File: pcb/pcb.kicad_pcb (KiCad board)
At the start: 2 copper layers, 49 x 31 mm, 37 parts, among them J1 Conn_02x08_Odd_Even, J2 B2B-PH-K-S_LF__SN_, J3 USB_C_Receptacle, J4 Conn_01x04, Q1 MMUN2211LT1G, SW1 SW_SPST, U1 TPS61090, U2 MCP73871-1AA

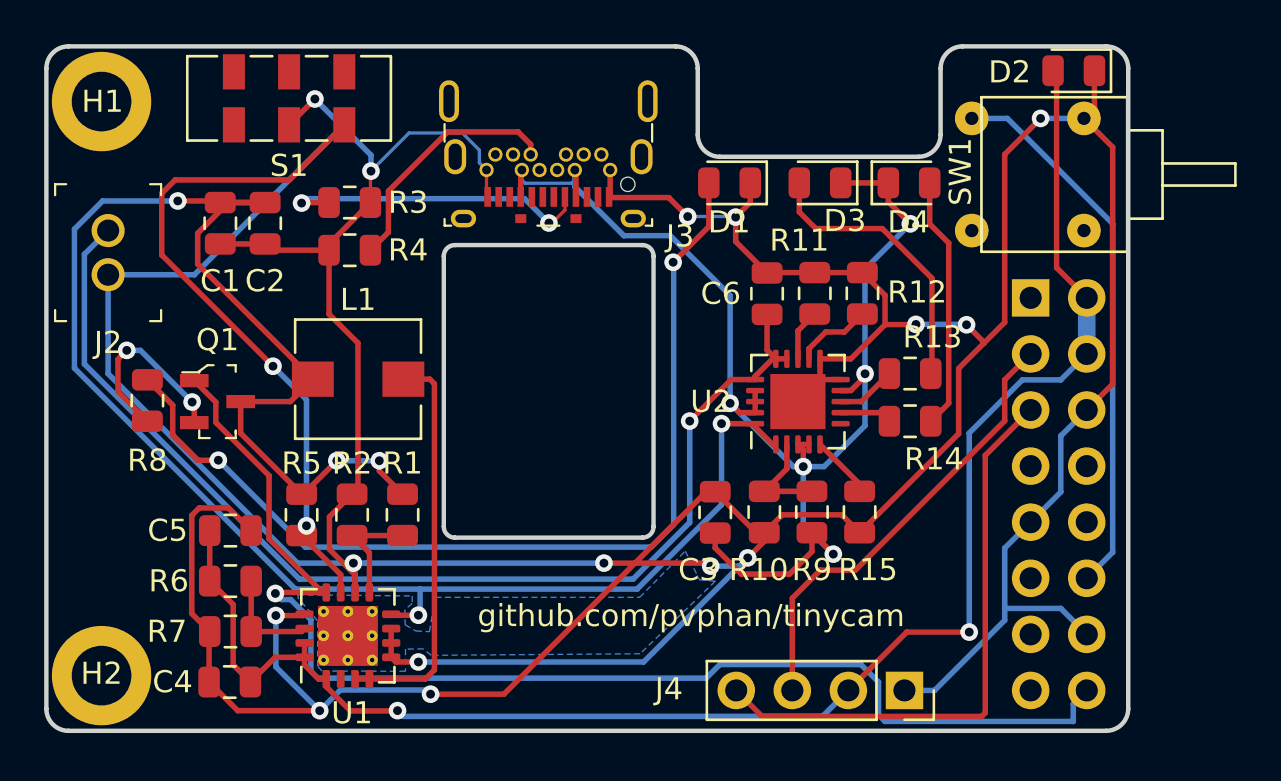
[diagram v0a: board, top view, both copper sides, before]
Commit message: revd to v1.1
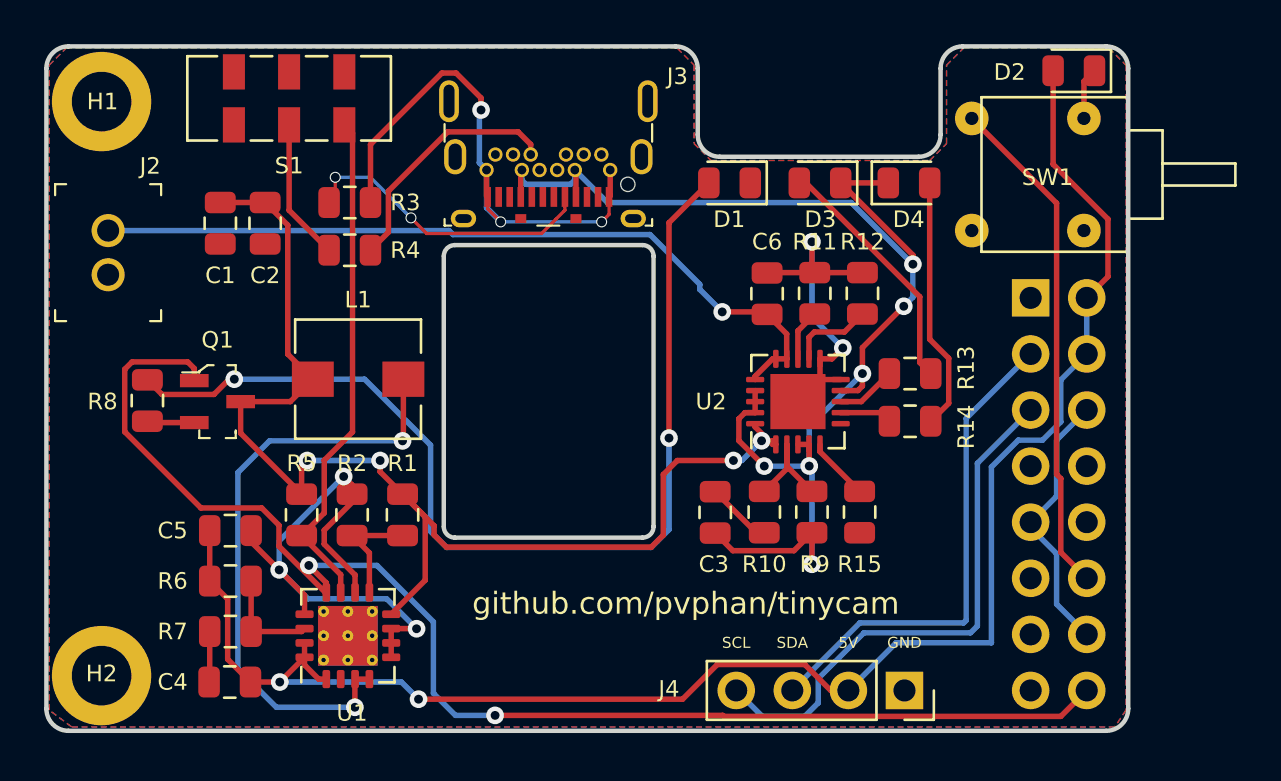
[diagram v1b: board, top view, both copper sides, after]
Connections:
- U1 pad 17: Net-(U1-Pad17) -> GND
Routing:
- net GND: track 259.9 -> 93.7 mm, vias 15 -> 8
- net VBAT: track 87.1 -> 56.6 mm, vias 5 -> 4
- net Net-(C6-Pad1): track 51.4 -> 35.9 mm
- net Net-(L1-Pad2): track 18.2 -> 27.7 mm, vias 0 -> 2
- net Net-(R5-Pad2): track 30.6 -> 23.0 mm, vias 2 -> 0
- net Net-(Q1-Pad2): track 8.83 -> 2.15 mm, vias 2 -> 0
- net PI_BCM_23: track 57.4 -> 61.5 mm, vias 1 -> 2
- net 5.0V: track 73.7 -> 77.1 mm
- net Net-(D1-Pad2): track 44.3 -> 46.4 mm
- net PI_BCM_18_PWM0: track 24.9 -> 23.0 mm
- net PI_BCM_3_SCL: track 26.4 -> 24.5 mm
- net PI_BCM_2_SDA: track 20.6 -> 22.5 mm
- net Net-(D3-Pad2): track 12.9 -> 11.3 mm
- net Net-(J3-PadA5): track 14.6 -> 13.8 mm
- net VBUS: track 61.2 -> 61.9 mm, vias 5 -> 6
- added copper zone on B.Cu, net GND
- added copper zone on F.Cu, net GND
- removed copper zone on B.Cu, net Net-(U1-Pad2)
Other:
- board text added: "5V"
- board text added: "GND"
- board text added: "SCL"
- board text added: "SDA"
